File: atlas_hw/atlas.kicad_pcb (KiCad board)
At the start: 4 copper layers, 70 x 70 mm, 151 parts, among them J1 USB_B_Micro, J10 PSP_LCD, J2 DEBUG_STM, J3 PSP_TOUCH, J5 CELL, J6 47352-1001, J7 DEBUG_STM, J9 PSP_LCD_BL, Q1 DMC2990UDJ, SW1 BTN_L, SW2 BTN_BOOT, SW3 ResetSTM, SW4 BTN_R, SW5 ResetNCP, SW7 BTN_C, U1 STM32H723VGT6, U10 MAX17048, U11 L96-M33, U12 LV52204MU, U14 MS5637, U18 FXOS8700CQ, U2 S27KL0641DABHV023, U3 MCP1810, U4 TLV62569DBV, U5 MX25L3233FM2I-08G, U6 ST1PS02, U7 EYSHSNZWZ, U8 MCP1640B, U9 BQ25606, Y1 8M, Y4 32k

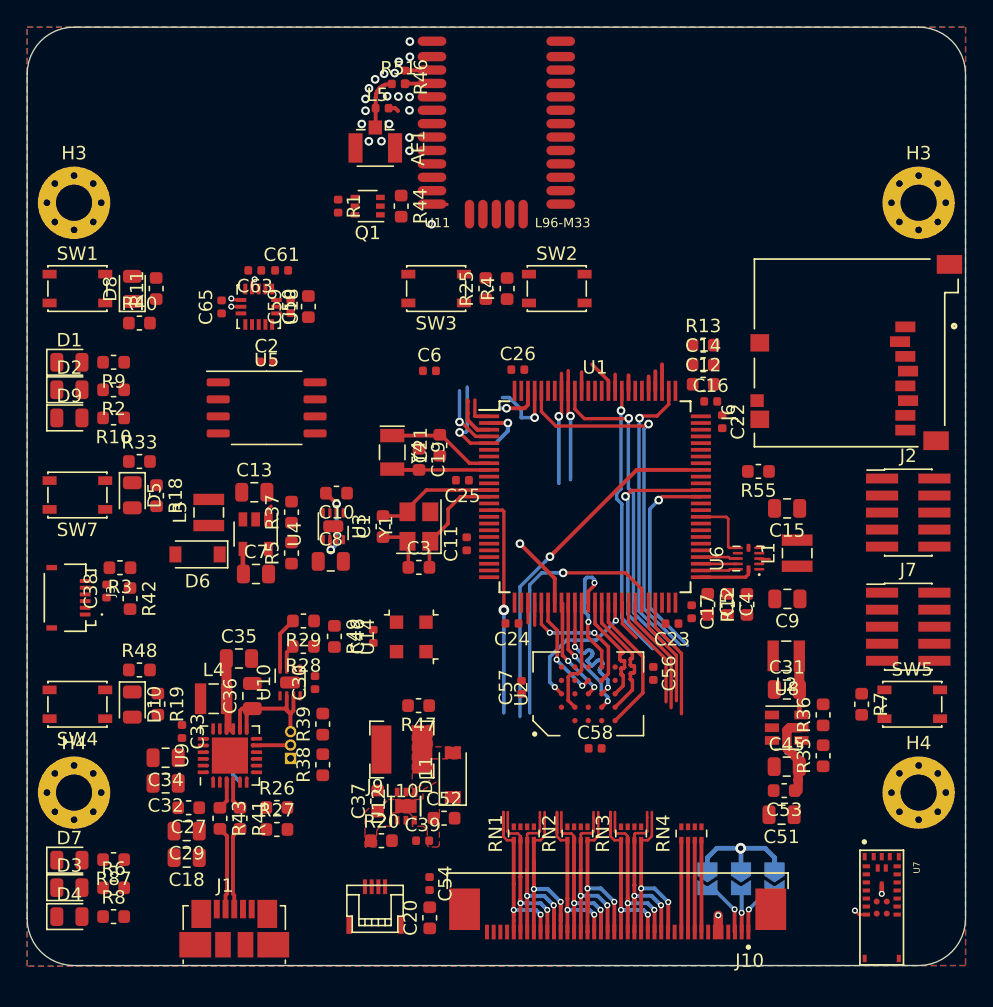
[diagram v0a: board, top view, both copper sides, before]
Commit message: layout done
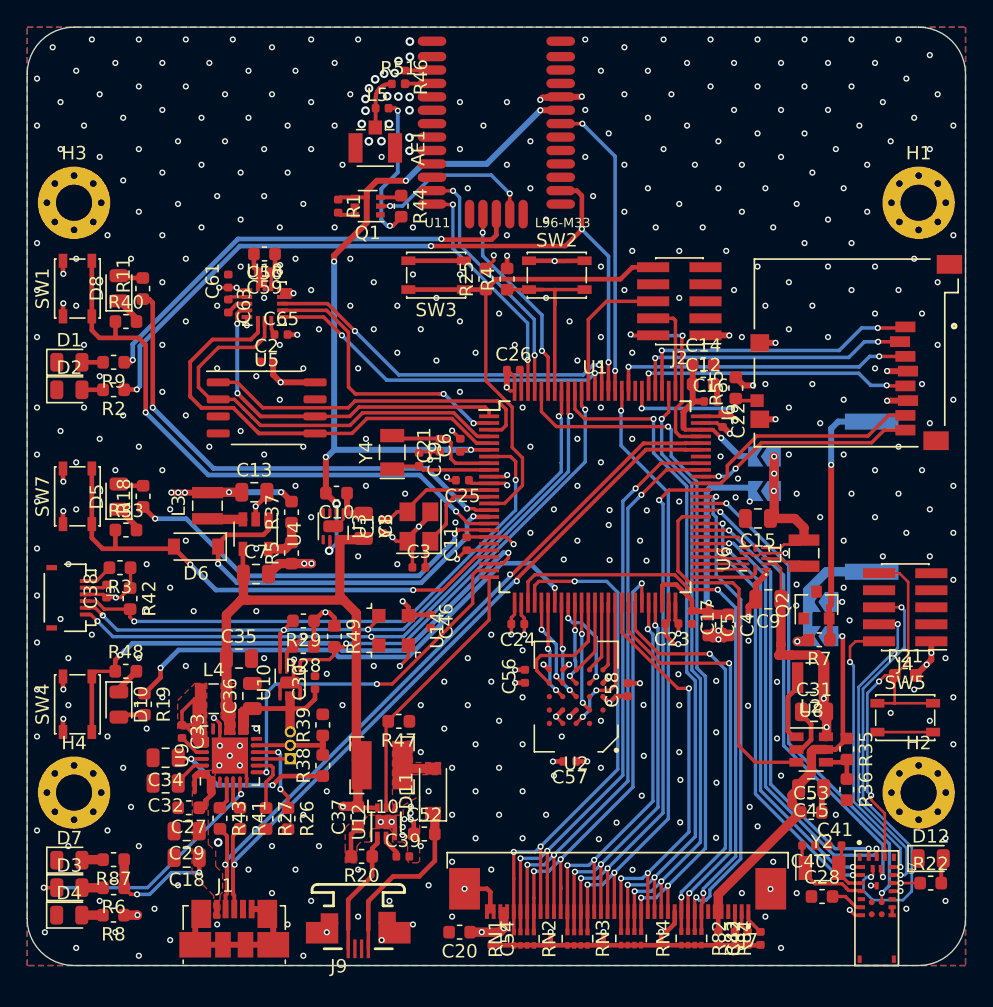
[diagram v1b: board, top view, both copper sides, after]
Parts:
- removed C51: 10u, Capacitor_SMD:C_0805_2012Metric
- removed D9: NCP_STATUS, LED_SMD:LED_0805_2012Metric
- removed the H3 at (100.2, 103.1)
- removed the H4 at (100.2, 147.1)
- removed J10: PSP_LCD, atlas:J_SMD_4-1734839-0-40_0.5_25.43_5.1_2.05
- removed R10: 1k, Resistor_SMD:R_0603_1608Metric
- added BZ1: Buzzer, atlas:PKLCS1212, B.Cu at (96.7, 125.0)
- added C28: 1u, Capacitor_SMD:C_0603_1608Metric, F.Cu at (92.9, 154.8)
- added C40: 18p, Capacitor_SMD:C_0402_1005Metric, F.Cu at (91.9, 151.0)
- added C41: 18p, Capacitor_SMD:C_0402_1005Metric, F.Cu at (93.9, 151.0)
- added C42: 0.1u, Capacitor_SMD:C_0402_1005Metric, F.Cu at (85.2, 158.0)
- added D12: NCP_0, LED_SMD:LED_0805_2012Metric, F.Cu at (101.0, 152.0)
- added G***: LOGO, atlas:europeart, B.Cu at (68.8, 125.0)
- added H1: MountingHole, MountingHole:MountingHole_2.7mm_M2.5_Pad_Via, F.Cu at (100.2, 103.1)
- added H2: MountingHole, MountingHole:MountingHole_2.7mm_M2.5_Pad_Via, F.Cu at (100.2, 147.1)
- added J4: DEBUG_NCP, Connector_PinHeader_1.27mm:PinHeader_2x05_P1.27mm_Vertical_SMD, F.Cu at (99.2, 133.3)
- added Q2: Q_NPN_BCE, Package_TO_SOT_SMD:SOT-23, F.Cu at (92.5, 133.1)
- added R14: 0, Jumper:SolderJumper-2_P1.3mm_Open_TrianglePad1.0x1.5mm, B.Cu at (92.9, 132.9)
- added R15: NP, Jumper:SolderJumper-2_P1.3mm_Open_TrianglePad1.0x1.5mm, B.Cu at (92.9, 135.4)
- added R21: 100k, Resistor_SMD:R_0603_1608Metric, F.Cu at (99.2, 138.3)
- added R22: 1k, Resistor_SMD:R_0603_1608Metric, F.Cu at (101.0, 153.8)
- added Y2: 32k, Crystal:Crystal_SMD_MicroCrystal_CC7V-T1A-2Pin_3.2x1.5mm, F.Cu at (92.9, 152.7)
- C1, C19, C21, C3: footprint Capacitor_SMD:C_0603_1608Metric -> Capacitor_SMD:C_0402_1005Metric
- J7: value DEBUG_STM -> Conn_01x40_Shielded; footprint Connector_PinHeader_1.27mm:PinHeader_2x05_P1.27mm_Vertical_SMD -> atlas:J_SMD_4-1734839-0-40_0.5_25.43_5.1_2.05
- J9: footprint atlas:Kyocera_046298_004_1x04_P0.5mm_Bottom -> atlas:SFV4R-1STE1LF
- R12, R13: footprint Resistor_SMD:R_0603_1608Metric -> Jumper:SolderJumper-2_P1.3mm_Open_TrianglePad1.0x1.5mm; moved to B.Cu
- R7: value 100k -> 1k
- R82, R83, R84: footprint Jumper:SolderJumper-2_P1.3mm_Open_TrianglePad1.0x1.5mm -> Resistor_SMD:R_0402_1005Metric; moved to F.Cu
- moved J7 30.4 mm to (77.7, 156.0), turned to 180 degrees
- moved J2 23.2 mm to (82.3, 110.5), turned to 180 degrees
- moved C56 9.59 mm to (70.8, 138.4), turned to 90 degrees
- moved R13 9.48 mm to (88.7, 122.0), turned to 180 degrees
- moved R12 8.56 mm to (88.7, 124.6), turned to 180 degrees
- moved RN1 7.85 mm to (70.7, 158.0)
- moved RN2 7.85 mm to (74.7, 158.0)
- moved RN3 7.82 mm to (78.7, 158.0)
- moved RN4 7.82 mm to (83.2, 158.0)
- moved C57 6.59 mm to (74.1, 144.8), turned to 180 degrees
- moved R55 6.44 mm to (86.5, 116.9), turned to 90 degrees
- moved C54 6.20 mm to (68.3, 158.0)
- moved C6 6.01 mm to (66.0, 121.2), turned to 90 degrees
- moved R36 5.85 mm to (94.8, 146.9), turned to 270 degrees
- moved R7 5.75 mm to (92.7, 135.7), turned to 180 degrees
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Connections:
- net /SD_VSEL renamed Net-(U1-Pad82)
- C9 pad 1: /VCC_3V3_MCU -> /VCC_SYS
- J7 pad 1: /VCC_3V3_MCU -> Net-(J7-Pad1)
- J7 pad 10: /DEBUG_NRESET_NCP -> /LTDC_DE
- J7 pad 2: /DEBUG_SWDIO_NCP -> Net-(J7-Pad2)
- J7 pad 3: GND -> Net-(J7-Pad3)
- J7 pad 4: /DEBUG_SWDCLK_NCP -> Net-(J7-Pad4)
- J7 pad 5: GND -> /VCC_LCD_PWR
- J7 pad 6: /DEBUG_SWO_NCP -> /VCC_LCD_PWR
- J7 pad 8: Net-(J7-Pad8) -> /LTDC_VS
- J7 pad 9: GND -> /LTDC_HS
- R12 pad 1: /VCAP1 -> /VCC_CORE
- R12 pad 2: /VCC_CORE -> /VCAP1
- R13 pad 1: /VCAP2 -> /VCC_CORE
- R13 pad 2: /VCC_CORE -> /VCAP2
- R20 pad 1: Net-(J9-Pad1) -> Net-(J9-Pad4)
- R28 pad 1: /VCC_3V3 -> /VCC_3V3_MCU
- R29 pad 1: /VCC_3V3 -> /VCC_3V3_MCU
- R42 pad 1: /VCC_3V3 -> /VCC_3V3_MCU
- R49 pad 1: /VCC_3V3 -> /VCC_3V3_MCU
- R7 pad 1: /DEBUG_NRESET_NCP -> Net-(BZ1-Pad2)
- R7 pad 2: /VCC_3V3_MCU -> Net-(BZ1-Pad1)
- R82 pad 2: Net-(J10-Pad3) -> Net-(J7-Pad3)
- R83 pad 2: Net-(J10-Pad2) -> Net-(J7-Pad2)
- R84 pad 2: Net-(J10-Pad1) -> Net-(J7-Pad1)
- RN1 pad 1: /LTDC_R4 -> GND
- RN1 pad 2: /LTDC_R5 -> GND
- RN1 pad 3: /LTDC_R6 -> GND
- RN1 pad 4: /LTDC_R7 -> GND
- RN1 pad 5: GND -> /LTDC_R7
- RN1 pad 6: GND -> /LTDC_R6
- RN1 pad 7: GND -> /LTDC_R5
- RN1 pad 8: GND -> /LTDC_R4
- RN2 pad 1: /LTDC_G4 -> GND
- RN2 pad 2: /LTDC_G5 -> GND
- RN2 pad 3: /LTDC_G6 -> GND
- RN2 pad 4: /LTDC_G7 -> GND
- RN2 pad 5: GND -> /LTDC_G7
- RN2 pad 6: GND -> /LTDC_G6
- RN2 pad 7: GND -> /LTDC_G5
- RN2 pad 8: GND -> /LTDC_G4
- RN3 pad 1: /LTDC_B4 -> GND
- RN3 pad 2: /LTDC_B5 -> GND
- RN3 pad 3: /LTDC_B6 -> GND
- RN3 pad 4: /LTDC_B7 -> GND
- RN3 pad 5: GND -> /LTDC_B7
- RN3 pad 6: GND -> /LTDC_B6
- RN3 pad 7: GND -> /LTDC_B5
- RN3 pad 8: GND -> /LTDC_B4
- RN4 pad 1: /LTDC_CK -> GND
- RN4 pad 2: /LTDC_DE -> GND
- RN4 pad 3: /LTDC_HS -> GND
- RN4 pad 4: /LTDC_VS -> GND
- RN4 pad 5: GND -> /LTDC_VS
- RN4 pad 6: GND -> /LTDC_HS
- RN4 pad 7: GND -> /LTDC_DE
- RN4 pad 8: GND -> /LTDC_CK
- SW1 pad 1: /VCC_MCU_3V3 -> /VCC_3V3_MCU
- SW2 pad 1: /VCC_MCU_3V3 -> /VCC_3V3_MCU
- SW4 pad 1: /VCC_MCU_3V3 -> /VCC_3V3_MCU
- SW7 pad 1: /VCC_MCU_3V3 -> /VCC_3V3_MCU
- U1 pad 15: /LTDC_R5 -> /STM_STATUS_L
- U1 pad 18: /SW_R -> /STM_STATUS_C
- U1 pad 2: /STM_STATUS_L -> /SPI4_ACCEL_NCS
- U1 pad 22: /JOY_X -> /SW_C_PWR
- U1 pad 23: /JOY_Y -> /SW_R
- U1 pad 57: /LCD_REG_EN -> /STM_VCORE_GOOD
- U1 pad 60: /STM_VCORE_GOOD -> /LCD_REG_EN
- U1 pad 61: /GPS_INT -> /PD14_NCP
- U1 pad 62: /GPS_FORCE_ON -> /PD15_NCP
- U1 pad 68: /LPUART1_TX_GPS -> /LTDC_R5
- U1 pad 69: /LPUART1_RX_GPS -> /BUZZER_T1C3
- U1 pad 7: /SW_PWR -> /TOUCH_INT
- U1 pad 85: /ACCEL_INT2 -> /GPS_INT
- U1 pad 86: /ACCEL_INT1 -> /GPS_3DF
- U1 pad 87: /FUEL_INT -> /ACCEL_INT1
- U1 pad 88: /TOUCH_INT -> /ACCEL_INT2
- U1 pad 90: /GYRO_INT -> /FUEL_INT
- U1 pad 95: /SDMMC1_CKIN -> /GPS_FORCEON
- U1 pad 97: /SPI4_ACCEL_NCS -> /GPS_UART8_RX
- U1 pad 98: /SPI4_GYRO_NCS -> /GPS_UART8_TX
- U11 pad 23: /VCC_3V3_MCU -> Net-(U11-Pad23)
- U11 pad 25: /LPUART1_RX_GPS -> /GPS_UART8_RX
- U11 pad 26: /LPUART1_TX_GPS -> /GPS_UART8_TX
- U11 pad 28: /GPS_FORCE_ON -> /GPS_FORCEON
- U12 pad 1: Net-(J9-Pad1) -> Net-(J9-Pad4)
- U2 pad A4: /DEBUG_NRESET_STM -> /VCC_3V3_MCU
- U6 pad 2: /VCC_3V3_MCU -> /VCC_SYS
- U7 pad 15: Net-(U7-Pad15) -> /NCP_STATUS_0
- U7 pad 19: Net-(U7-Pad19) -> /DEBUG_NRESET_NCP
- U7 pad 2: Net-(U7-Pad2) -> /USART3_TX_NCP
- U7 pad 20: Net-(U7-Pad20) -> /USART3_RX_NCP
- U7 pad 21: Net-(U7-Pad21) -> /USART3_CTS_NCP
- U7 pad 22: Net-(U7-Pad22) -> /DEBUG_SWO_NCP
- U7 pad 24: Net-(U7-Pad24) -> /PD15_NCP
- U7 pad 25: /DEBUG_NRESET_NCP -> /PD14_NCP
- U7 pad 3: Net-(U7-Pad3) -> /USART3_RTS_NCP
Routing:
- net GND: track 13.4 -> 158.7 mm, vias 21 -> 480
- net /VCC_SYS: track 14.7 -> 127.7 mm, vias 0 -> 3
- net /VCC_3V3_MCU: track 0.97 -> 88.5 mm, vias 1 -> 45
- net /GPS_3DF: track 0.00 -> 58.7 mm, vias 0 -> 4
- net /VCC_BACKUP: track 6.21 -> 62.0 mm, vias 3 -> 7
- net /USB_PORT_D+: track 6.25 -> 57.4 mm, vias 0 -> 2
- net /USB_PORT_D-: track 6.24 -> 56.6 mm, vias 0 -> 2
- net /SW_L: track 0.00 -> 45.0 mm, vias 0 -> 2
- net /TOUCH_INT: track 0.00 -> 42.3 mm, vias 0 -> 2
- net /SW_R: track 0.00 -> 42.0 mm, vias 0 -> 2
- net /I2C4_SCL_SENSOR: track 10.1 -> 51.9 mm, vias 1 -> 4
- net /I2C4_SDA_SENSOR: track 12.3 -> 52.6 mm, vias 1 -> 4
- net /SW_C_PWR: track 0.00 -> 38.9 mm, vias 0 -> 2
- net /DEBUG_NRESET_STM: track 0.00 -> 37.9 mm
- net /PD15_NCP: track 0.00 -> 36.9 mm, vias 0 -> 2
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- added copper zone on F.Cu, net /USB_PORT_VBUS
- added copper zone on F.Cu, net /VCC_SYS
- added copper zone on F.Cu, net Net-(C33-Pad1)
